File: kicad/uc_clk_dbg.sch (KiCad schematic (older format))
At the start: 17 parts, among them J601 pin header 2x6 2.54, U301 TMS320F28388DZWTS, U602 M25PX32-VMW, Y601 26mhz

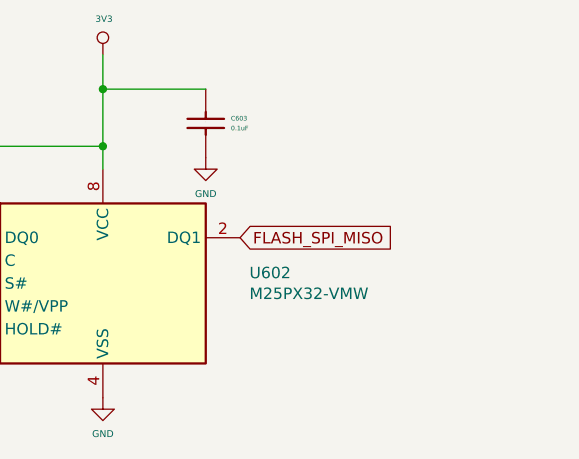
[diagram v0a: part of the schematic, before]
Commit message: stackup
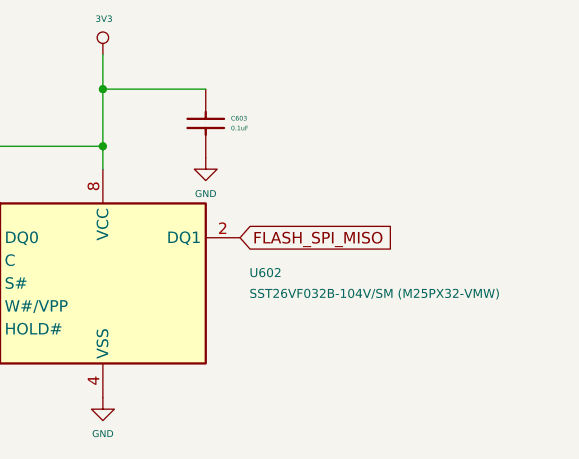
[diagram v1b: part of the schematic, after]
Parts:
- C601, C602, C603: price@10 (none) -> 0.05800
- D603, D604: digikey LB Q39G-L2OO-35-1 -> 475-2816-1-ND; price@10 (none) -> 0.40100
- U602: value M25PX32-VMW -> SST26VF032B-104V/SM (M25PX32-VMW); Description (none) -> FLASH Memory IC 32Mb (4M x 8) SPI - Quad I/O 104MHz 8-SOIJ; PartNumber (none) -> SST26VF032B-104V/SM; digikey (none) -> SST26VF032B-104V/SM-ND; price@10 (none) -> 1.67000
- Y601: value 26mhz -> osc 25Mhz; Description (none) -> 25MHz XO (Standard) HCMOS Oscillator 3.3V Enable/Disable 4-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; PartNumber (none) -> ECS-2520S33-250-FN-TR; digikey (none) -> XC2198CT-ND; price@10 (none) -> 1.41900
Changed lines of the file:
@@
 F 4 "311-1335-1-ND" H 0   0   50  0001 C CNN "digikey"
 F 5 "CAP CER 0.1UF 16V X7R 0603 " H 0   0   50  0001 C CNN "Description"
-F 6 "" H 0   0   50  0001 C CNN "Mfr part number"
-F 7 "CC0603KPX7R7BB104" H 0   0   50  0001 C CNN "PartNumber"
+F 6 "CC0603KPX7R7BB104" H 0   0   50  0001 C CNN "PartNumber"
+F 7 "0.05800" H 0   0   50  0001 C CNN "price@10"
 	1    13900 3800
 	0    -1   -1   0
@@
 P 13900 2600
 F 0 "Y601" H 13900 2367 60  0000 C CNN
-F 1 "26mhz" H 13900 2600 50  0001 C CNN
+F 1 "osc 25Mhz" H 13900 2600 50  0001 C CNN
 F 2 "servo:Crystal_SMD_2520-4Pin_2.5x2.0mm" H 13900 2600 50  0001 C CNN
 F 3 "../doc/datasheets//ECS-2520S.pdf" H 13900 2600 50  0001 C CNN
+F 4 "25MHz XO (Standard) HCMOS Oscillator 3.3V Enable/Disable 4-SMD, No Lead " H 0   0   50  0001 C CNN "Description"
+F 5 "ECS-2520S33-250-FN-TR" H 0   0   50  0001 C CNN "PartNumber"
+F 6 "XC2198CT-ND " H 0   0   50  0001 C CNN "digikey"
+F 7 "1.41900" H 0   0   50  0001 C CNN "price@10"
 	1    13900 2600
 	-1   0    0    -1
@@
 F 2 "servo:LED_0603_1608Metric" H 4200 3050 60  0001 C CNN
 F 3 "../doc/datasheets/LB_Q39G_v1.4_9-1-15.pdf" H 4200 3050 60  0001 C CNN
-F 4 "LB Q39G-L2OO-35-1" H 4400 3250 50  0001 C CNN "digikey"
+F 4 "475-2816-1-ND" H 4400 3250 50  0001 C CNN "digikey"
 F 5 "LB Q39G-L2OO-35-1" H 0   0   50  0001 C CNN "PartNumber"
 F 6 "LED BLUE DIFFUSED 0603 SMD " H 0   0   50  0001 C CNN "Description"
+F 7 "0.40100" H 0   0   50  0001 C CNN "price@10"
 	1    4400 3250
 	0    1    1    0
@@
 F 2 "servo:LED_0603_1608Metric" H 8050 3250 60  0001 C CNN
 F 3 "../doc/datasheets/LB_Q39G_v1.4_9-1-15.pdf" H 8050 3250 60  0001 C CNN
-F 4 "LB Q39G-L2OO-35-1" H 8250 3450 50  0001 C CNN "digikey"
+F 4 "475-2816-1-ND" H 8250 3450 50  0001 C CNN "digikey"
 F 5 "LB Q39G-L2OO-35-1" H 0   0   50  0001 C CNN "PartNumber"
 F 6 "LED BLUE DIFFUSED 0603 SMD " H 0   0   50  0001 C CNN "Description"
+F 7 "0.40100" H 0   0   50  0001 C CNN "price@10"
 	1    8250 3450
 	0    1    1    0
@@
 F 4 "311-1335-1-ND" H 0   0   50  0001 C CNN "digikey"
 F 5 "CAP CER 0.1UF 16V X7R 0603 " H 0   0   50  0001 C CNN "Description"
-F 6 "" H 0   0   50  0001 C CNN "Mfr part number"
-F 7 "CC0603KPX7R7BB104" H 0   0   50  0001 C CNN "PartNumber"
+F 6 "CC0603KPX7R7BB104" H 0   0   50  0001 C CNN "PartNumber"
+F 7 "0.05800" H 0   0   50  0001 C CNN "price@10"
 	1    14300 7250
 	0    1    1    0
@@
 U 1 1 5ECE67BA
 P 13850 8000
-F 0 "U602" H 14491 8046 50  0000 L CNN
-F 1 "M25PX32-VMW" H 14491 7955 50  0000 L CNN
+F 0 "U602" H 14491 8046 39  0000 L CNN
+F 1 "SST26VF032B-104V/SM (M25PX32-VMW)" H 14491 7955 39  0000 L CNN
 F 2 "servo:SOIJ-8_5.3x5.3mm_P1.27mm" H 14500 8050 50  0001 C CNN
-F 3 "../doc/datasheets/m25px32.pdf" H 14000 7900 50  0001 C CNN
+F 3 "../doc/datasheets/SST26VF032B_nor_flash.pdf" H 14000 7900 50  0001 C CNN
+F 4 "FLASH Memory IC 32Mb (4M x 8) SPI - Quad I/O 104MHz 8-SOIJ" H 0   0   50  0001 C CNN "Description"
+F 5 "SST26VF032B-104V/SM" H 0   0   50  0001 C CNN "PartNumber"
+F 6 "SST26VF032B-104V/SM-ND " H 0   0   50  0001 C CNN "digikey"
+F 7 "1.67000" H 0   0   50  0001 C CNN "price@10"
 	1    13850 8000
 	1    0    0    -1
@@
 F 5 "CC0603KPX7R7BB104" H 0   0   50  0001 C CNN "PartNumber"
 F 6 "311-1335-1-ND" H 0   0   50  0001 C CNN "digikey"
+F 7 "0.05800" H 0   0   50  0001 C CNN "price@10"
 	1    10300 7550
 	0    1    1    0
